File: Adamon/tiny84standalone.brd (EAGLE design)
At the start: 75.9 x 31.7 mm, 29 parts

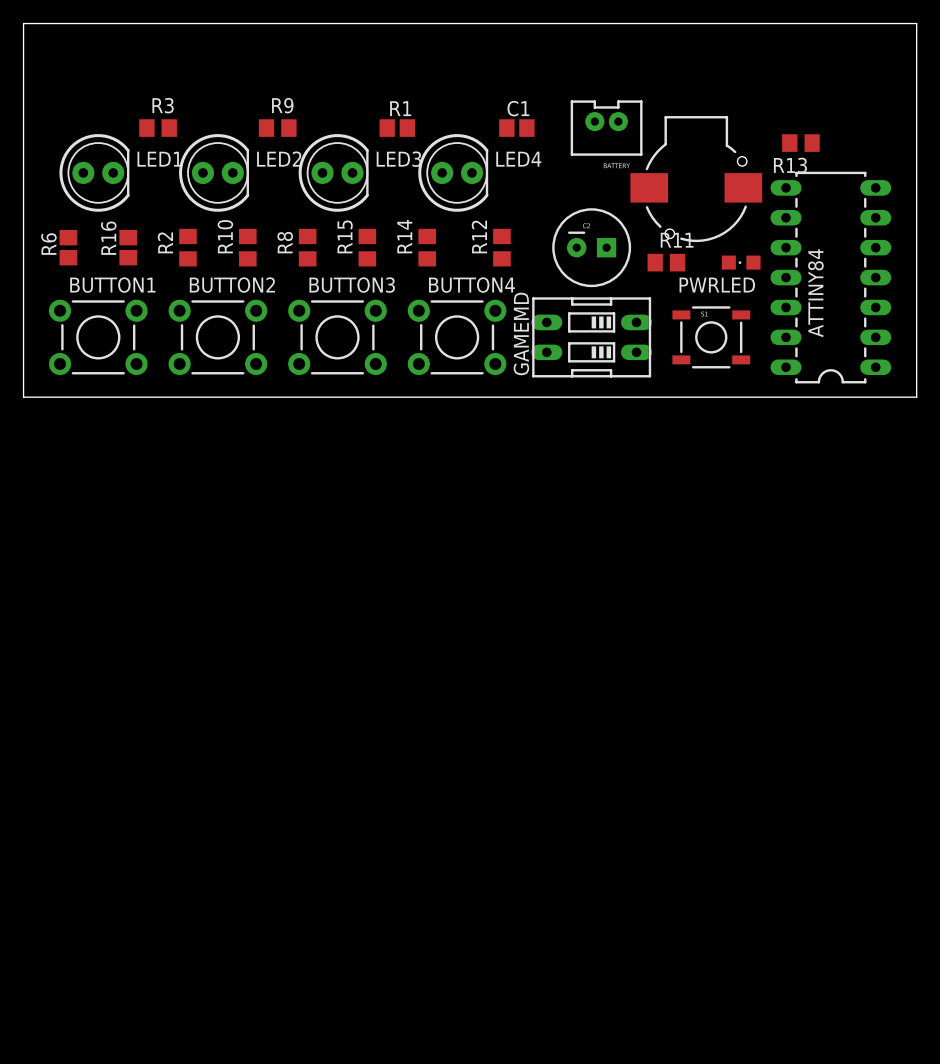
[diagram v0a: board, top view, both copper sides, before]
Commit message: awh yeah
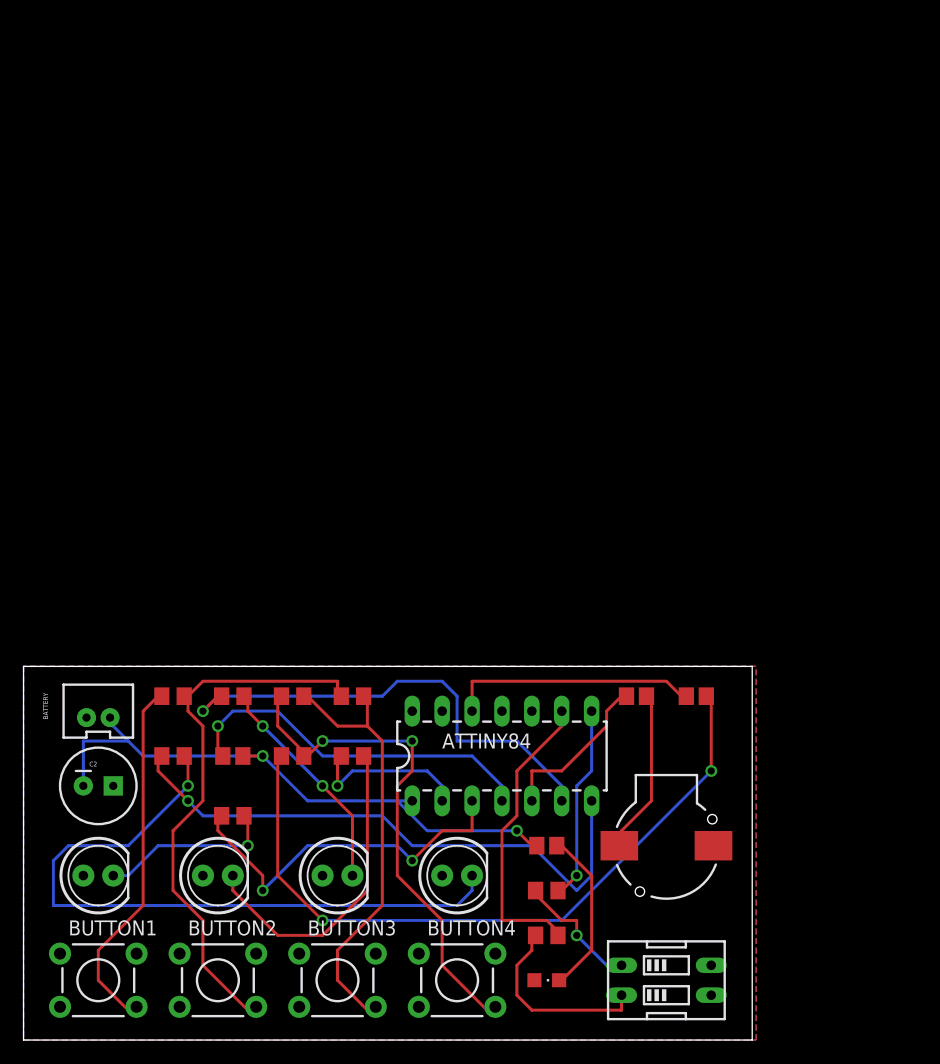
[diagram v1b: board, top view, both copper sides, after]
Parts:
- removed S1: RESET, SparkFun-Electromechanical:TACTILE_SWITCH_SMD
- moved R3 72.7 mm to (44.5, 12.7)
- moved R2 65.9 mm to (44.5, 8.89), turned to 0 degrees
- moved BATTERY 65.7 mm to (6.35, 27.9), turned to 0 degrees
- moved R6 65.1 mm to (44.5, 16.5), turned to 180 degrees
- moved R13 64.5 mm to (27.9, 24.1), turned to 0 degrees
- moved PWRLED 63.2 mm to (44.5, 5.08), turned to 270 degrees
- moved C2 62.0 mm to (6.35, 21.6)
- moved LED1 59.7 mm to (6.35, 14.0)
- moved LED2 59.7 mm to (16.5, 14.0)
- moved LED3 59.7 mm to (26.7, 14.0)
- moved LED4 59.7 mm to (36.8, 14.0)
- moved R16 57.6 mm to (52.1, 29.2), turned to 180 degrees
- moved BUZZER 55.9 mm to (54.6, 16.5)
- moved R1 55.1 mm to (17.8, 24.1)
- moved GAMEMD 55.0 mm to (54.6, 5.08), turned to 270 degrees
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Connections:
- net GND: no longer S1.2
- net N$5: no longer S1.4
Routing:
- net N$9: track 0.00 -> 60.9 mm, vias 0 -> 2
- net N$32: track 0.00 -> 58.1 mm, vias 0 -> 1
- net VCC: track 0.00 -> 51.5 mm, vias 0 -> 2
- net N$13: track 0.00 -> 49.5 mm, vias 0 -> 1
- net N$17: track 0.00 -> 46.8 mm
- net N$20: track 0.00 -> 43.5 mm, vias 0 -> 2
- net N$12: track 0.00 -> 40.8 mm, vias 0 -> 1
- net N$18: track 0.00 -> 37.4 mm
- net N$10: track 0.00 -> 31.7 mm, vias 0 -> 2
- net N$5: track 0.00 -> 31.5 mm, vias 0 -> 1
- net N$14: track 0.00 -> 30.9 mm
- net N$35: track 0.00 -> 27.6 mm
- net N$21: track 0.00 -> 25.8 mm
- net N$22: track 0.00 -> 21.3 mm
- net N$33: track 0.00 -> 19.2 mm, vias 0 -> 2
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- added copper zone on layer 1, net GND
- added copper zone on layer 16, net GND
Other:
- board size 75.9 x 31.7 mm -> 61.9 x 31.7 mm
